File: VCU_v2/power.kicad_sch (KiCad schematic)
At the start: 12 parts

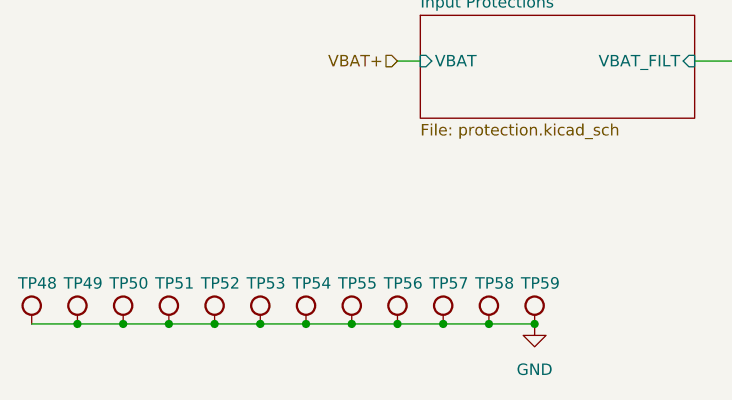
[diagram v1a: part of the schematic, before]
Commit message: vcu v2 schematics done
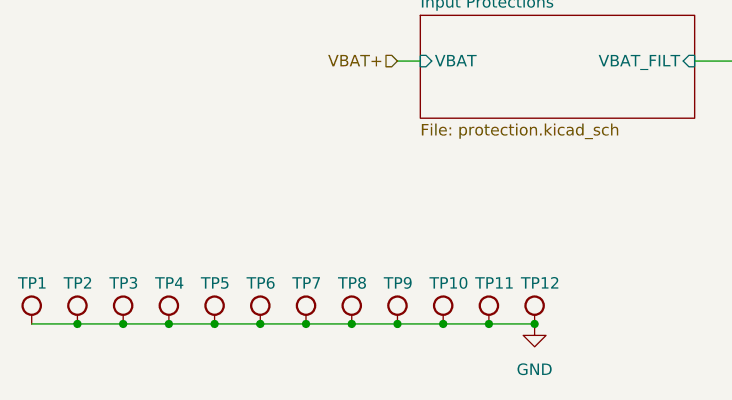
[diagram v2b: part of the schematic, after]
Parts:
- renumbered TP48 to TP1, TP57 to TP10, TP58 to TP11, TP59 to TP12, TP49 to TP2, TP50 to TP3, TP51 to TP4, TP52 to TP5, TP53 to TP6, TP54 to TP7, TP55 to TP8, TP56 to TP9
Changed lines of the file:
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@@
 		(on_board yes)
 		(dnp no)
-		(property "Reference" "TP50"
+		(property "Reference" "TP3"
 			(at 79.7568 119.2037 0)
 			(effects
@@
 			(project "VCU_v1"
 				(path "/4ee6c2ad-9a1b-4276-b3cf-1cc8dc52967e/9e4b5f8d-93dc-46d5-aa92-d0e0d2e07b3d"
-					(reference "TP50")
+					(reference "TP3")
 					(unit 1)
 				)
@@
 		(on_board yes)
 		(dnp no)
-		(property "Reference" "TP52"
+		(property "Reference" "TP5"
 			(at 89.9168 119.2037 0)
 			(effects
@@
 			(project "VCU_v1"
 				(path "/4ee6c2ad-9a1b-4276-b3cf-1cc8dc52967e/9e4b5f8d-93dc-46d5-aa92-d0e0d2e07b3d"
-					(reference "TP52")
+					(reference "TP5")
 					(unit 1)
 				)
@@
 		(dnp no)
 		(fields_autoplaced yes)
-		(property "Reference" "#PWR0144"
+		(property "Reference" "#PWR06"
 			(at 127 130.81 0)
 			(effects
@@
 			(project ""
 				(path "/4ee6c2ad-9a1b-4276-b3cf-1cc8dc52967e/9e4b5f8d-93dc-46d5-aa92-d0e0d2e07b3d"
-					(reference "#PWR0144")
+					(reference "#PWR06")
 					(unit 1)
 				)
@@
 		(dnp no)
 		(fields_autoplaced yes)
-		(property "Reference" "#PWR04"
+		(property "Reference" "#PWR05"
 			(at 104.14 68.58 0)
 			(effects
@@
 			(project ""
 				(path "/4ee6c2ad-9a1b-4276-b3cf-1cc8dc52967e/9e4b5f8d-93dc-46d5-aa92-d0e0d2e07b3d"
-					(reference "#PWR04")
+					(reference "#PWR05")
 					(unit 1)
 				)
@@
 		(on_board yes)
 		(dnp no)
-		(property "Reference" "TP57"
+		(property "Reference" "TP10"
 			(at 115.3168 119.2037 0)
 			(effects
@@
 			(project "VCU_v1"
 				(path "/4ee6c2ad-9a1b-4276-b3cf-1cc8dc52967e/9e4b5f8d-93dc-46d5-aa92-d0e0d2e07b3d"
-					(reference "TP57")
+					(reference "TP10")
 					(unit 1)
 				)
@@
 		(on_board yes)
 		(dnp no)
-		(property "Reference" "TP58"
+		(property "Reference" "TP11"
 			(at 120.3968 119.2037 0)
 			(effects
@@
 			(project "VCU_v1"
 				(path "/4ee6c2ad-9a1b-4276-b3cf-1cc8dc52967e/9e4b5f8d-93dc-46d5-aa92-d0e0d2e07b3d"
-					(reference "TP58")
+					(reference "TP11")
 					(unit 1)
 				)
@@
 		(on_board yes)
 		(dnp no)
-		(property "Reference" "TP59"
+		(property "Reference" "TP12"
 			(at 125.4768 119.2037 0)
 			(effects
@@
 			(project "VCU_v1"
 				(path "/4ee6c2ad-9a1b-4276-b3cf-1cc8dc52967e/9e4b5f8d-93dc-46d5-aa92-d0e0d2e07b3d"
-					(reference "TP59")
+					(reference "TP12")
 					(unit 1)
 				)
@@
 		(on_board yes)
 		(dnp no)
-		(property "Reference" "TP54"
+		(property "Reference" "TP7"
 			(at 100.0768 119.2037 0)
 			(effects
@@
 			(project "VCU_v1"
 				(path "/4ee6c2ad-9a1b-4276-b3cf-1cc8dc52967e/9e4b5f8d-93dc-46d5-aa92-d0e0d2e07b3d"
-					(reference "TP54")
+					(reference "TP7")
 					(unit 1)
 				)
@@
 		(on_board yes)
 		(dnp no)
-		(property "Reference" "TP51"
+		(property "Reference" "TP4"
 			(at 84.8368 119.2037 0)
 			(effects
@@
 			(project "VCU_v1"
 				(path "/4ee6c2ad-9a1b-4276-b3cf-1cc8dc52967e/9e4b5f8d-93dc-46d5-aa92-d0e0d2e07b3d"
-					(reference "TP51")
+					(reference "TP4")
 					(unit 1)
 				)
@@
 		(on_board yes)
 		(dnp no)
-		(property "Reference" "TP48"
+		(property "Reference" "TP1"
 			(at 69.5968 119.2037 0)
 			(effects
@@
 			(project "VCU_v1"
 				(path "/4ee6c2ad-9a1b-4276-b3cf-1cc8dc52967e/9e4b5f8d-93dc-46d5-aa92-d0e0d2e07b3d"
-					(reference "TP48")
+					(reference "TP1")
 					(unit 1)
 				)
@@
 		(dnp no)
 		(fields_autoplaced yes)
-		(property "Reference" "#PWR09"
+		(property "Reference" "#PWR010"
 			(at 161.29 73.66 0)
 			(effects
@@
 			(project ""
 				(path "/4ee6c2ad-9a1b-4276-b3cf-1cc8dc52967e/9e4b5f8d-93dc-46d5-aa92-d0e0d2e07b3d"
-					(reference "#PWR09")
+					(reference "#PWR010")
 					(unit 1)
 				)
@@
 		(dnp no)
 		(fields_autoplaced yes)
-		(property "Reference" "#PWR05"
+		(property "Reference" "#PWR07"
 			(at 152.4 99.06 0)
 			(effects
@@
 			(project ""
 				(path "/4ee6c2ad-9a1b-4276-b3cf-1cc8dc52967e/9e4b5f8d-93dc-46d5-aa92-d0e0d2e07b3d"
-					(reference "#PWR05")
+					(reference "#PWR07")
 					(unit 1)
 				)
@@
 		(dnp no)
 		(fields_autoplaced yes)
-		(property "Reference" "#PWR03"
+		(property "Reference" "#PWR04"
 			(at 104.14 46.99 0)
 			(effects
@@
 			(project ""
 				(path "/4ee6c2ad-9a1b-4276-b3cf-1cc8dc52967e/9e4b5f8d-93dc-46d5-aa92-d0e0d2e07b3d"
-					(reference "#PWR03")
+					(reference "#PWR04")
 					(unit 1)
 				)
@@
 		(dnp no)
 		(fields_autoplaced yes)
-		(property "Reference" "#PWR07"
+		(property "Reference" "#PWR08"
 			(at 154.94 46.99 0)
 			(effects
@@
 			(project ""
 				(path "/4ee6c2ad-9a1b-4276-b3cf-1cc8dc52967e/9e4b5f8d-93dc-46d5-aa92-d0e0d2e07b3d"
-					(reference "#PWR07")
+					(reference "#PWR08")
 					(unit 1)
 				)
@@
 		(on_board yes)
 		(dnp no)
-		(property "Reference" "TP49"
+		(property "Reference" "TP2"
 			(at 74.6768 119.2037 0)
 			(effects
@@
 			(project "VCU_v1"
 				(path "/4ee6c2ad-9a1b-4276-b3cf-1cc8dc52967e/9e4b5f8d-93dc-46d5-aa92-d0e0d2e07b3d"
-					(reference "TP49")
+					(reference "TP2")
 					(unit 1)
 				)
@@
 		(on_board yes)
 		(dnp no)
-		(property "Reference" "TP56"
+		(property "Reference" "TP9"
 			(at 110.2368 119.2037 0)
 			(effects
@@
 			(project "VCU_v1"
 				(path "/4ee6c2ad-9a1b-4276-b3cf-1cc8dc52967e/9e4b5f8d-93dc-46d5-aa92-d0e0d2e07b3d"
-					(reference "TP56")
+					(reference "TP9")
 					(unit 1)
 				)
@@
 		(on_board yes)
 		(dnp no)
-		(property "Reference" "TP53"
+		(property "Reference" "TP6"
 			(at 94.9968 119.2037 0)
 			(effects
@@
 			(project "VCU_v1"
 				(path "/4ee6c2ad-9a1b-4276-b3cf-1cc8dc52967e/9e4b5f8d-93dc-46d5-aa92-d0e0d2e07b3d"
-					(reference "TP53")
+					(reference "TP6")
 					(unit 1)
 				)
@@
 		(on_board yes)
 		(dnp no)
-		(property "Reference" "TP55"
+		(property "Reference" "TP8"
 			(at 105.1568 119.2037 0)
 			(effects
@@
 			(project "VCU_v1"
 				(path "/4ee6c2ad-9a1b-4276-b3cf-1cc8dc52967e/9e4b5f8d-93dc-46d5-aa92-d0e0d2e07b3d"
-					(reference "TP55")
+					(reference "TP8")
 					(unit 1)
 				)
@@
 		(dnp no)
 		(fields_autoplaced yes)
-		(property "Reference" "#PWR08"
+		(property "Reference" "#PWR09"
 			(at 154.94 71.12 0)
 			(effects
@@
 			(project ""
 				(path "/4ee6c2ad-9a1b-4276-b3cf-1cc8dc52967e/9e4b5f8d-93dc-46d5-aa92-d0e0d2e07b3d"
-					(reference "#PWR08")
+					(reference "#PWR09")
 					(unit 1)
 				)

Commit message: placements friggin 80% friggin done shoutout epstein
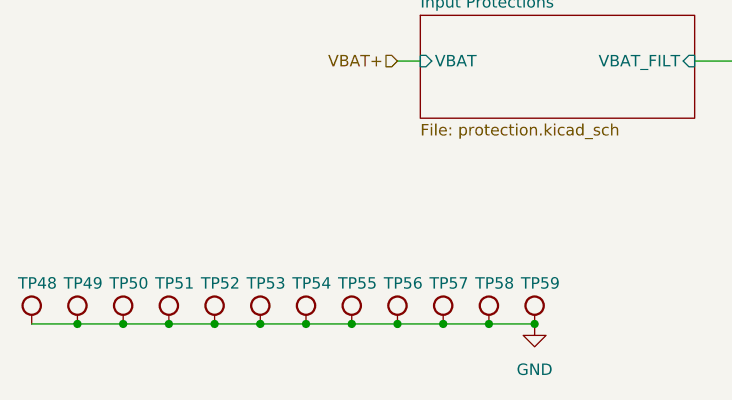
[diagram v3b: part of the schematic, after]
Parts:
- renumbered TP1 to TP48, TP2 to TP49, TP3 to TP50, TP4 to TP51, TP5 to TP52, TP6 to TP53, TP7 to TP54, TP8 to TP55, TP9 to TP56, TP10 to TP57, TP11 to TP58, TP12 to TP59
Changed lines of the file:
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@@
 		(on_board yes)
 		(dnp no)
-		(property "Reference" "TP3"
+		(property "Reference" "TP50"
 			(at 79.7568 119.2037 0)
 			(effects
@@
 			(project "VCU_v1"
 				(path "/4ee6c2ad-9a1b-4276-b3cf-1cc8dc52967e/9e4b5f8d-93dc-46d5-aa92-d0e0d2e07b3d"
-					(reference "TP3")
+					(reference "TP50")
 					(unit 1)
 				)
@@
 		(on_board yes)
 		(dnp no)
-		(property "Reference" "TP5"
+		(property "Reference" "TP52"
 			(at 89.9168 119.2037 0)
 			(effects
@@
 			(project "VCU_v1"
 				(path "/4ee6c2ad-9a1b-4276-b3cf-1cc8dc52967e/9e4b5f8d-93dc-46d5-aa92-d0e0d2e07b3d"
-					(reference "TP5")
+					(reference "TP52")
 					(unit 1)
 				)
@@
 		(dnp no)
 		(fields_autoplaced yes)
-		(property "Reference" "#PWR06"
+		(property "Reference" "#PWR0144"
 			(at 127 130.81 0)
 			(effects
@@
 			(project ""
 				(path "/4ee6c2ad-9a1b-4276-b3cf-1cc8dc52967e/9e4b5f8d-93dc-46d5-aa92-d0e0d2e07b3d"
-					(reference "#PWR06")
+					(reference "#PWR0144")
 					(unit 1)
 				)
@@
 		(dnp no)
 		(fields_autoplaced yes)
-		(property "Reference" "#PWR05"
+		(property "Reference" "#PWR04"
 			(at 104.14 68.58 0)
 			(effects
@@
 			(project ""
 				(path "/4ee6c2ad-9a1b-4276-b3cf-1cc8dc52967e/9e4b5f8d-93dc-46d5-aa92-d0e0d2e07b3d"
-					(reference "#PWR05")
+					(reference "#PWR04")
 					(unit 1)
 				)
@@
 		(on_board yes)
 		(dnp no)
-		(property "Reference" "TP10"
+		(property "Reference" "TP57"
 			(at 115.3168 119.2037 0)
 			(effects
@@
 			(project "VCU_v1"
 				(path "/4ee6c2ad-9a1b-4276-b3cf-1cc8dc52967e/9e4b5f8d-93dc-46d5-aa92-d0e0d2e07b3d"
-					(reference "TP10")
+					(reference "TP57")
 					(unit 1)
 				)
@@
 		(on_board yes)
 		(dnp no)
-		(property "Reference" "TP11"
+		(property "Reference" "TP58"
 			(at 120.3968 119.2037 0)
 			(effects
@@
 			(project "VCU_v1"
 				(path "/4ee6c2ad-9a1b-4276-b3cf-1cc8dc52967e/9e4b5f8d-93dc-46d5-aa92-d0e0d2e07b3d"
-					(reference "TP11")
+					(reference "TP58")
 					(unit 1)
 				)
@@
 		(on_board yes)
 		(dnp no)
-		(property "Reference" "TP12"
+		(property "Reference" "TP59"
 			(at 125.4768 119.2037 0)
 			(effects
@@
 			(project "VCU_v1"
 				(path "/4ee6c2ad-9a1b-4276-b3cf-1cc8dc52967e/9e4b5f8d-93dc-46d5-aa92-d0e0d2e07b3d"
-					(reference "TP12")
+					(reference "TP59")
 					(unit 1)
 				)
@@
 		(on_board yes)
 		(dnp no)
-		(property "Reference" "TP7"
+		(property "Reference" "TP54"
 			(at 100.0768 119.2037 0)
 			(effects
@@
 			(project "VCU_v1"
 				(path "/4ee6c2ad-9a1b-4276-b3cf-1cc8dc52967e/9e4b5f8d-93dc-46d5-aa92-d0e0d2e07b3d"
-					(reference "TP7")
+					(reference "TP54")
 					(unit 1)
 				)
@@
 		(on_board yes)
 		(dnp no)
-		(property "Reference" "TP4"
+		(property "Reference" "TP51"
 			(at 84.8368 119.2037 0)
 			(effects
@@
 			(project "VCU_v1"
 				(path "/4ee6c2ad-9a1b-4276-b3cf-1cc8dc52967e/9e4b5f8d-93dc-46d5-aa92-d0e0d2e07b3d"
-					(reference "TP4")
+					(reference "TP51")
 					(unit 1)
 				)
@@
 		(on_board yes)
 		(dnp no)
-		(property "Reference" "TP1"
+		(property "Reference" "TP48"
 			(at 69.5968 119.2037 0)
 			(effects
@@
 			(project "VCU_v1"
 				(path "/4ee6c2ad-9a1b-4276-b3cf-1cc8dc52967e/9e4b5f8d-93dc-46d5-aa92-d0e0d2e07b3d"
-					(reference "TP1")
+					(reference "TP48")
 					(unit 1)
 				)
@@
 		(dnp no)
 		(fields_autoplaced yes)
-		(property "Reference" "#PWR010"
+		(property "Reference" "#PWR09"
 			(at 161.29 73.66 0)
 			(effects
@@
 			(project ""
 				(path "/4ee6c2ad-9a1b-4276-b3cf-1cc8dc52967e/9e4b5f8d-93dc-46d5-aa92-d0e0d2e07b3d"
-					(reference "#PWR010")
+					(reference "#PWR09")
 					(unit 1)
 				)
@@
 		(dnp no)
 		(fields_autoplaced yes)
-		(property "Reference" "#PWR07"
+		(property "Reference" "#PWR05"
 			(at 152.4 99.06 0)
 			(effects
@@
 			(project ""
 				(path "/4ee6c2ad-9a1b-4276-b3cf-1cc8dc52967e/9e4b5f8d-93dc-46d5-aa92-d0e0d2e07b3d"
-					(reference "#PWR07")
+					(reference "#PWR05")
 					(unit 1)
 				)
@@
 		(dnp no)
 		(fields_autoplaced yes)
-		(property "Reference" "#PWR04"
+		(property "Reference" "#PWR03"
 			(at 104.14 46.99 0)
 			(effects
@@
 			(project ""
 				(path "/4ee6c2ad-9a1b-4276-b3cf-1cc8dc52967e/9e4b5f8d-93dc-46d5-aa92-d0e0d2e07b3d"
-					(reference "#PWR04")
+					(reference "#PWR03")
 					(unit 1)
 				)
@@
 		(dnp no)
 		(fields_autoplaced yes)
-		(property "Reference" "#PWR08"
+		(property "Reference" "#PWR07"
 			(at 154.94 46.99 0)
 			(effects
@@
 			(project ""
 				(path "/4ee6c2ad-9a1b-4276-b3cf-1cc8dc52967e/9e4b5f8d-93dc-46d5-aa92-d0e0d2e07b3d"
-					(reference "#PWR08")
+					(reference "#PWR07")
 					(unit 1)
 				)
@@
 		(on_board yes)
 		(dnp no)
-		(property "Reference" "TP2"
+		(property "Reference" "TP49"
 			(at 74.6768 119.2037 0)
 			(effects
@@
 			(project "VCU_v1"
 				(path "/4ee6c2ad-9a1b-4276-b3cf-1cc8dc52967e/9e4b5f8d-93dc-46d5-aa92-d0e0d2e07b3d"
-					(reference "TP2")
+					(reference "TP49")
 					(unit 1)
 				)
@@
 		(on_board yes)
 		(dnp no)
-		(property "Reference" "TP9"
+		(property "Reference" "TP56"
 			(at 110.2368 119.2037 0)
 			(effects
@@
 			(project "VCU_v1"
 				(path "/4ee6c2ad-9a1b-4276-b3cf-1cc8dc52967e/9e4b5f8d-93dc-46d5-aa92-d0e0d2e07b3d"
-					(reference "TP9")
+					(reference "TP56")
 					(unit 1)
 				)
@@
 		(on_board yes)
 		(dnp no)
-		(property "Reference" "TP6"
+		(property "Reference" "TP53"
 			(at 94.9968 119.2037 0)
 			(effects
@@
 			(project "VCU_v1"
 				(path "/4ee6c2ad-9a1b-4276-b3cf-1cc8dc52967e/9e4b5f8d-93dc-46d5-aa92-d0e0d2e07b3d"
-					(reference "TP6")
+					(reference "TP53")
 					(unit 1)
 				)
@@
 		(on_board yes)
 		(dnp no)
-		(property "Reference" "TP8"
+		(property "Reference" "TP55"
 			(at 105.1568 119.2037 0)
 			(effects
@@
 			(project "VCU_v1"
 				(path "/4ee6c2ad-9a1b-4276-b3cf-1cc8dc52967e/9e4b5f8d-93dc-46d5-aa92-d0e0d2e07b3d"
-					(reference "TP8")
+					(reference "TP55")
 					(unit 1)
 				)
@@
 		(dnp no)
 		(fields_autoplaced yes)
-		(property "Reference" "#PWR09"
+		(property "Reference" "#PWR08"
 			(at 154.94 71.12 0)
 			(effects
@@
 			(project ""
 				(path "/4ee6c2ad-9a1b-4276-b3cf-1cc8dc52967e/9e4b5f8d-93dc-46d5-aa92-d0e0d2e07b3d"
-					(reference "#PWR09")
+					(reference "#PWR08")
 					(unit 1)
 				)
